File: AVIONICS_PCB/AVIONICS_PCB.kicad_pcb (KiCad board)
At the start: 2 copper layers, 38 x 145.4 mm, 14 parts, among them IC1 MMBT2222ALT1G, IC2 MMBT2222ALT1G, J1 XT30PW-M, J2 Screw_Terminal_01x02, J3 Screw_Terminal_01x02, U1 ESP32-S3-DevKitC

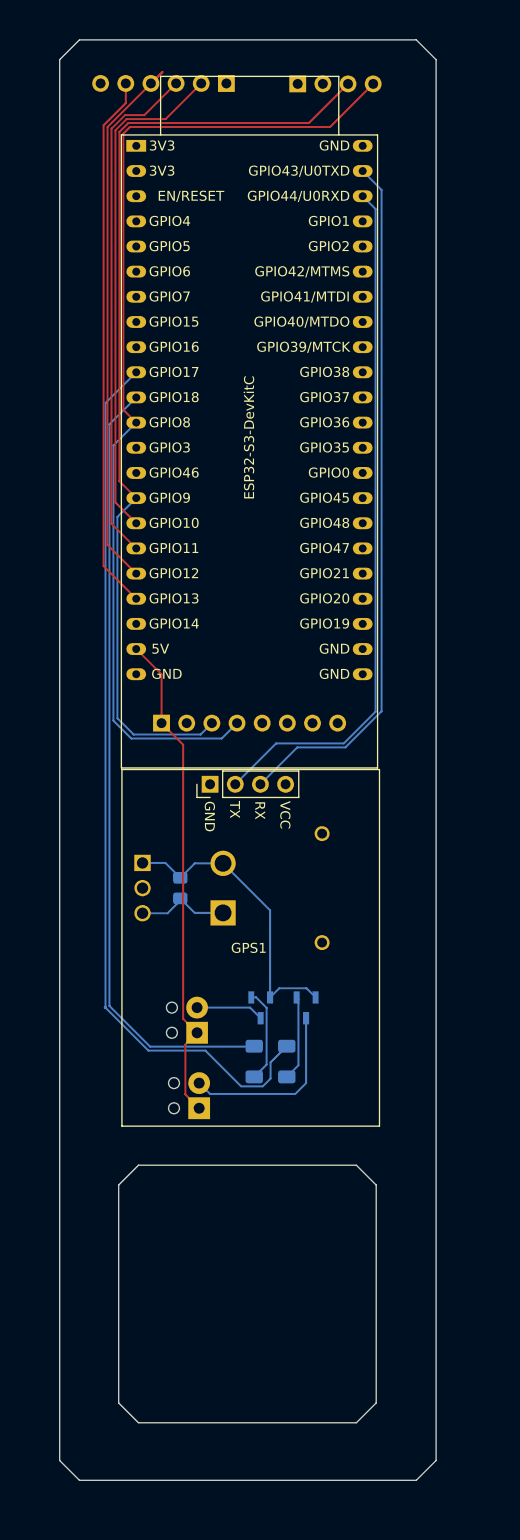
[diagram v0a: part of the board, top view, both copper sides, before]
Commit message: Board v2
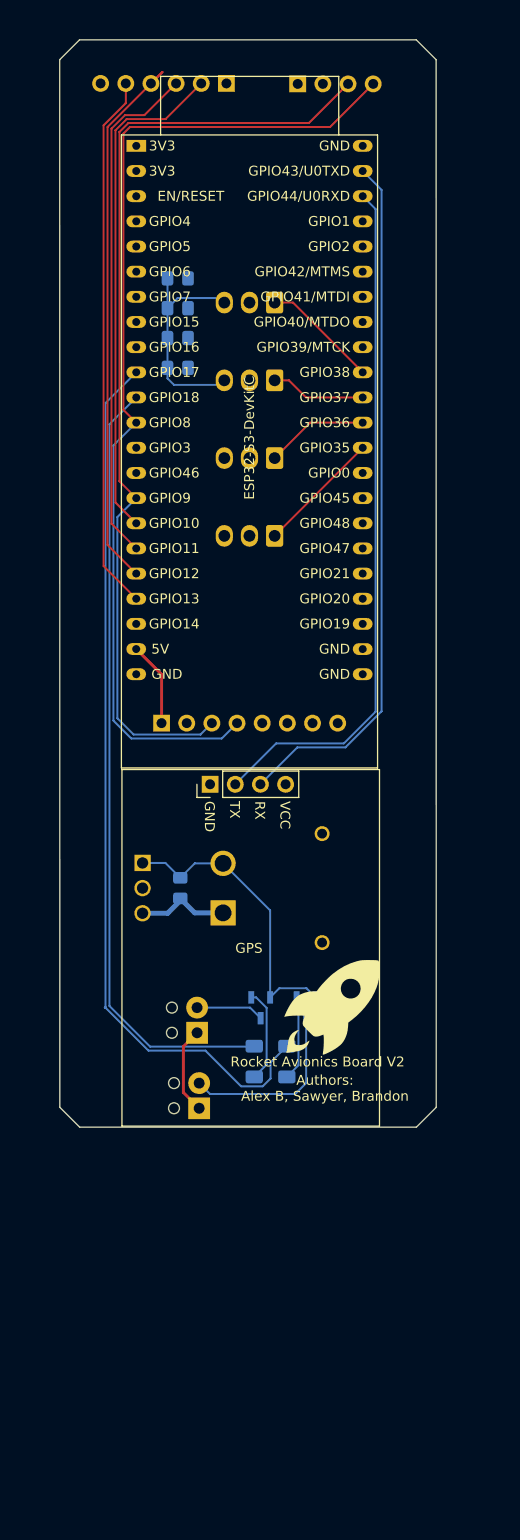
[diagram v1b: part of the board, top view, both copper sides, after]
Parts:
- added C2: C, Capacitor_SMD:C_0805_2012Metric_Pad1.18x1.45mm_HandSolder, B.Cu at (144.5, 54.0)
- added C3: C, Capacitor_SMD:C_0805_2012Metric_Pad1.18x1.45mm_HandSolder, B.Cu at (144.5, 57.0)
- added C4: C, Capacitor_SMD:C_0805_2012Metric_Pad1.18x1.45mm_HandSolder, B.Cu at (144.5, 60.0)
- added C5: C, Capacitor_SMD:C_0805_2012Metric_Pad1.18x1.45mm_HandSolder, B.Cu at (144.5, 63.0)
- added G***: LOGO, LOGO, F.Cu at (160.0, 127.6)
- added J4: Conn_01x03, Connector_Molex:Molex_KK-254_AE-6410-03A_1x03_P2.54mm_Vertical, B.Cu at (154.3, 56.5)
- added J5: Conn_01x03, Connector_Molex:Molex_KK-254_AE-6410-03A_1x03_P2.54mm_Vertical, B.Cu at (154.3, 64.3)
- added J6: Conn_01x03, Connector_Molex:Molex_KK-254_AE-6410-03A_1x03_P2.54mm_Vertical, B.Cu at (154.3, 72.2)
- added J7: Conn_01x03, Connector_Molex:Molex_KK-254_AE-6410-03A_1x03_P2.54mm_Vertical, B.Cu at (154.3, 80.0)
- renumbered ACCELEROMETER1 to ACCELEROMETER, ALTITUDE1 to ALTITUDE, GPS1 to GPS, SD_READER1 to SD_READER
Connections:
- J1 pad S1: (no net) -> GND
- J1 pad S2: (no net) -> GND
- J2 pad 1: +5V -> +3V3
- J3 pad 1: +5V -> +3V3
- U1 pad 32: unconnected-(U1-GPIO35-Pad32) -> servo4
- U1 pad 33: unconnected-(U1-GPIO36-Pad33) -> servo3
- U1 pad 34: unconnected-(U1-GPIO37-Pad34) -> servo2
- U1 pad 35: unconnected-(U1-GPIO38-Pad35) -> servo1
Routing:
- net +5V: track 50.0 -> 8.54 mm
- net GND: track 30.2 -> 52.9 mm
- net servo4: track 0.00 -> 12.6 mm
- net servo1: track 0.00 -> 11.8 mm
- net servo3: track 0.00 -> 10.4 mm
- net servo2: track 0.00 -> 9.61 mm
- net +3V3: track 0.00 -> 8.85 mm
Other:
- board size 38 x 145.4 mm -> 38 x 109.8 mm
- board text added: "Authors: Alex B, Sawyer, Brandon"
- board text added: "Rocket Avionics Board V2"
